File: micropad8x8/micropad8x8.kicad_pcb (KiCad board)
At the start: 2 copper layers, 262.6 x 185.5 mm, 49 parts, among them U1 Raspberry_Pi_Pico

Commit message: Added logo and smaller base
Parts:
- removed the REF** at (272.4, 99.2)
- removed the REF** at (158.1, 99.2)
- removed the REF** at (100.3, 18.2)
- removed the REF** at (21.7, 113.2)
- removed the REF** at (102.7, 194.1)
- removed the REF** at (133.6, 99.2)
- removed the REF** at (21.7, 194.1)
- removed the REF** at (239.1, 99.2)
- removed the REF** at (239.1, 18.2)
- removed the REF** at (272.4, 18.2)
- removed the REF** at (133.6, 18.2)
- removed the REF** at (158.1, 18.2)
- removed the REF** at (102.7, 113.2)
- removed the REF** at (19.3, 99.2)
- added REF**: OSHW-Logo2_14.6x12mm_SilkScreen, Symbol:OSHW-Logo2_14.6x12mm_SilkScreen, F.Cu at (116.3, 79.3)
- added REF**: MountingHole_3.2mm_M3_Pad_TopBottom, MountingHole:MountingHole_3.2mm_M3_Pad_TopBottom, F.Cu at (99.7, 112.2)
- added REF**: MountingHole_3.2mm_M3_Pad_TopBottom, MountingHole:MountingHole_3.2mm_M3_Pad_TopBottom, F.Cu at (100.3, 18.2)
- added REF**: MountingHole_3.2mm_M3_Pad_TopBottom, MountingHole:MountingHole_3.2mm_M3_Pad_TopBottom, F.Cu at (18.8, 112.2)
- added REF**: MountingHole_3.2mm_M3_Pad_TopBottom, MountingHole:MountingHole_3.2mm_M3_Pad_TopBottom, F.Cu at (99.7, 193.2)
- added REF**: MountingHole_3.2mm_M3_Pad_TopBottom, MountingHole:MountingHole_3.2mm_M3_Pad_TopBottom, F.Cu at (246.7, 18.2)
- added REF**: MountingHole_3.2mm_M3_Pad_TopBottom, MountingHole:MountingHole_3.2mm_M3_Pad_TopBottom, F.Cu at (132.3, 99.2)
- added REF**: MountingHole_3.2mm_M3_Pad_TopBottom, MountingHole:MountingHole_3.2mm_M3_Pad_TopBottom, F.Cu at (131.7, 193.2)
- added REF**: MountingHole_3.2mm_M3_Pad_TopBottom, MountingHole:MountingHole_3.2mm_M3_Pad_TopBottom, F.Cu at (18.8, 193.2)
- added REF**: MountingHole_3.2mm_M3_Pad_TopBottom, MountingHole:MountingHole_3.2mm_M3_Pad_TopBottom, F.Cu at (165.8, 18.2)
- added REF**: MountingHole_3.2mm_M3_Pad_TopBottom, MountingHole:MountingHole_3.2mm_M3_Pad_TopBottom, F.Cu at (131.7, 112.2)
- added REF**: MountingHole_3.2mm_M3_Pad_TopBottom, MountingHole:MountingHole_3.2mm_M3_Pad_TopBottom, F.Cu at (132.3, 18.2)
- added REF**: MountingHole_3.2mm_M3_Pad_TopBottom, MountingHole:MountingHole_3.2mm_M3_Pad_TopBottom, F.Cu at (19.3, 99.2)
- added REF**: MountingHole_3.2mm_M3_Pad_TopBottom, MountingHole:MountingHole_3.2mm_M3_Pad_TopBottom, F.Cu at (246.7, 99.2)
- added REF**: MountingHole_3.2mm_M3_Pad_TopBottom, MountingHole:MountingHole_3.2mm_M3_Pad_TopBottom, F.Cu at (165.8, 99.2)
- moved U1 0.70 mm to (116.3, 41.4)
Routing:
- net Row 3: track 94.8 -> 96.6 mm
- net Row 0: track 81.1 -> 82.5 mm
- net Col 0: track 143.3 -> 142.8 mm
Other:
- board size 262.6 x 185.5 mm -> 236 x 183 mm
- board text added: "Nibell Macropad 4x4 16 v1.0 2023 https://github.com/Nibell"

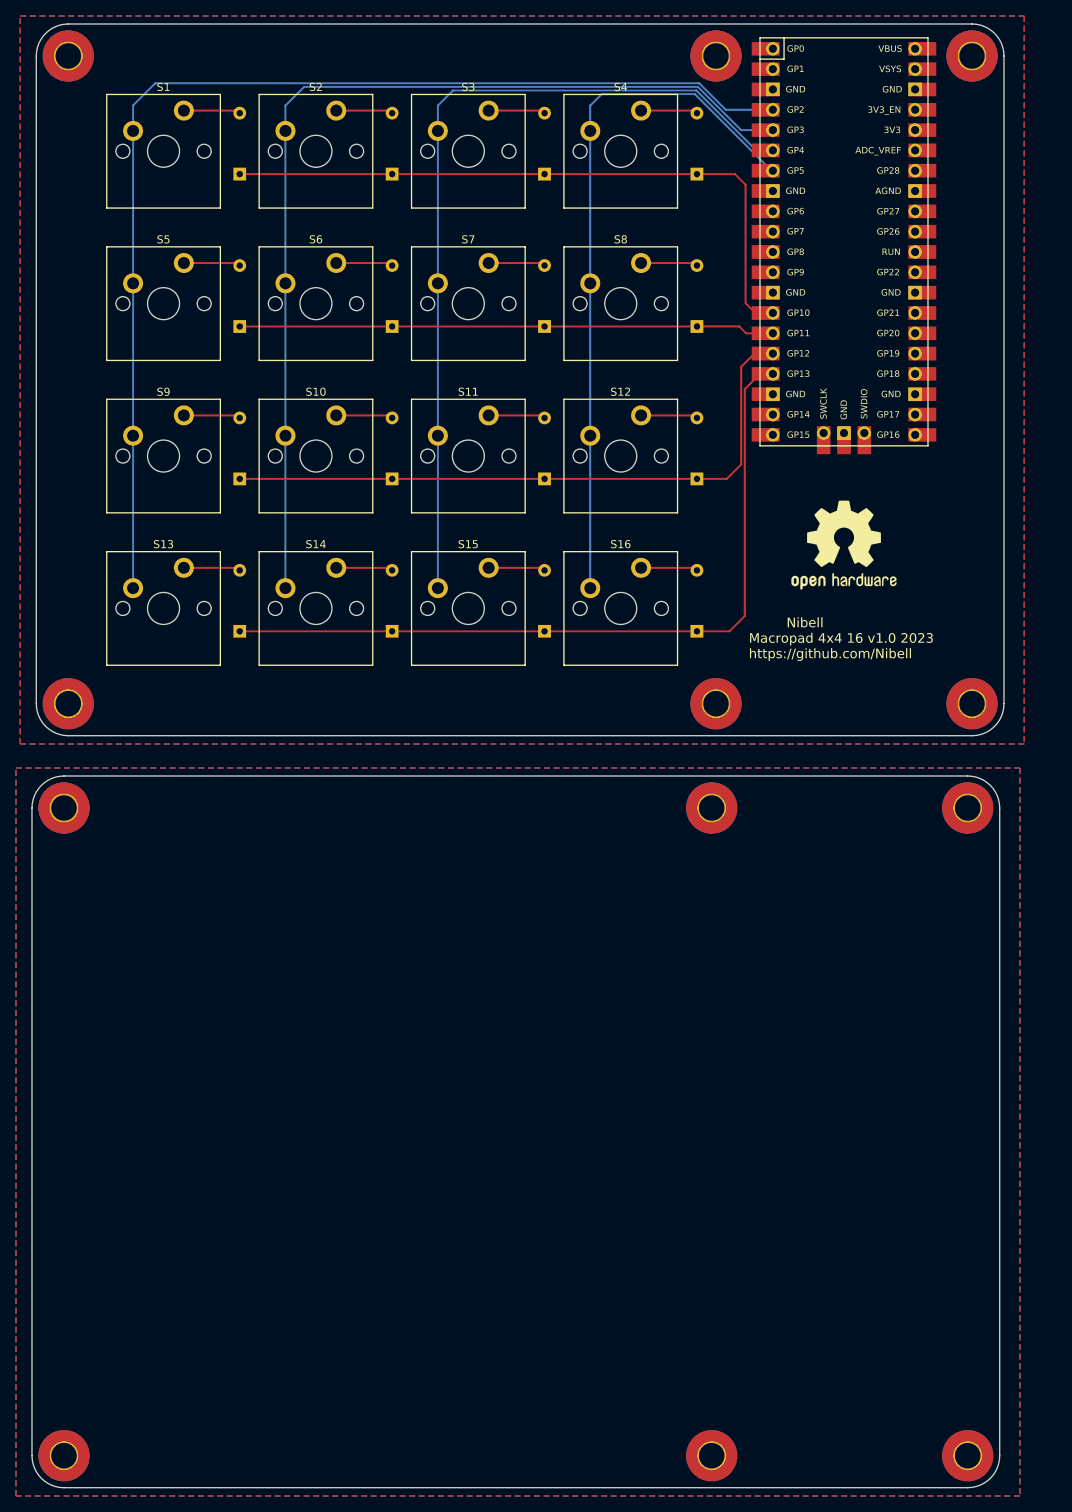
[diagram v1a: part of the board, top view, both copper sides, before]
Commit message: final version
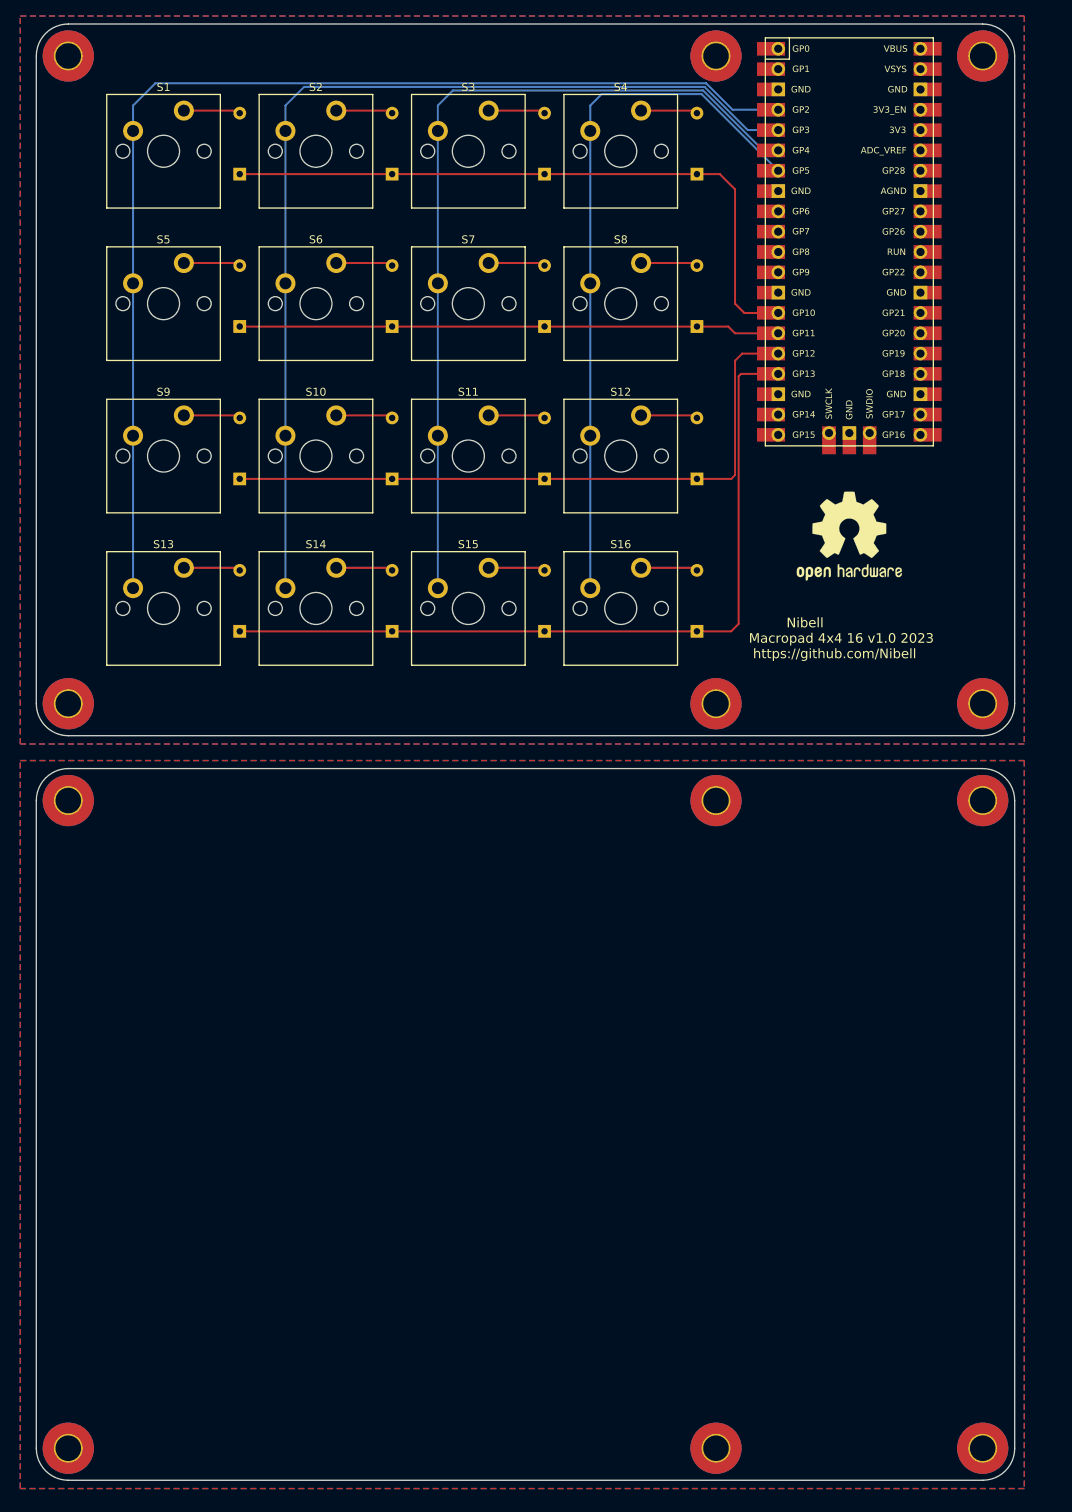
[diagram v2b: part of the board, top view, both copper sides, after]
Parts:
- removed the REF** at (99.7, 112.2)
- removed the REF** at (18.8, 112.2)
- removed the REF** at (99.7, 193.2)
- removed the REF** at (131.7, 193.2)
- removed the REF** at (18.8, 193.2)
- removed the REF** at (131.7, 112.2)
- added REF**: MountingHole_3.2mm_M3_Pad_TopBottom, MountingHole:MountingHole_3.2mm_M3_Pad_TopBottom, F.Cu at (133.6, 111.3)
- added REF**: MountingHole_3.2mm_M3_Pad_TopBottom, MountingHole:MountingHole_3.2mm_M3_Pad_TopBottom, F.Cu at (100.3, 111.3)
- added REF**: MountingHole_3.2mm_M3_Pad_TopBottom, MountingHole:MountingHole_3.2mm_M3_Pad_TopBottom, F.Cu at (19.3, 192.2)
- added REF**: MountingHole_3.2mm_M3_Pad_TopBottom, MountingHole:MountingHole_3.2mm_M3_Pad_TopBottom, F.Cu at (19.3, 111.3)
- added REF**: MountingHole_3.2mm_M3_Pad_TopBottom, MountingHole:MountingHole_3.2mm_M3_Pad_TopBottom, F.Cu at (100.3, 192.2)
- added REF**: MountingHole_3.2mm_M3_Pad_TopBottom, MountingHole:MountingHole_3.2mm_M3_Pad_TopBottom, F.Cu at (133.6, 192.2)
- moved REF** 1.34 mm to (133.6, 99.2)
- moved REF** 1.34 mm to (133.6, 18.2)
- moved REF** 1.31 mm to (116.9, 78.2)
- moved U1 0.67 mm to (116.9, 41.4)
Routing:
- net Row 3: track 96.6 -> 98.8 mm
- net Row 2: track 80.3 -> 82.2 mm
- net Row 1: track 67.3 -> 68.0 mm
- net Col 0: track 142.8 -> 143.5 mm
- net Col 3: track 87.7 -> 88.4 mm
- net Col 2: track 106.1 -> 106.7 mm
- net Col 1: track 124.5 -> 125.1 mm
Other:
- board size 236 x 183 mm -> 235.4 x 182 mm
- board text removed: "MountingHole_3.2mm_M3_Pad_TopBottom"
